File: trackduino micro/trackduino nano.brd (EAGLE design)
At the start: 48.1 x 21.9 mm, 28 parts, among them IC2 74AHC1G125DBV, SW1 SPST_TACT-KMR2, U1 ATMEGA168, Y1 16MHZ

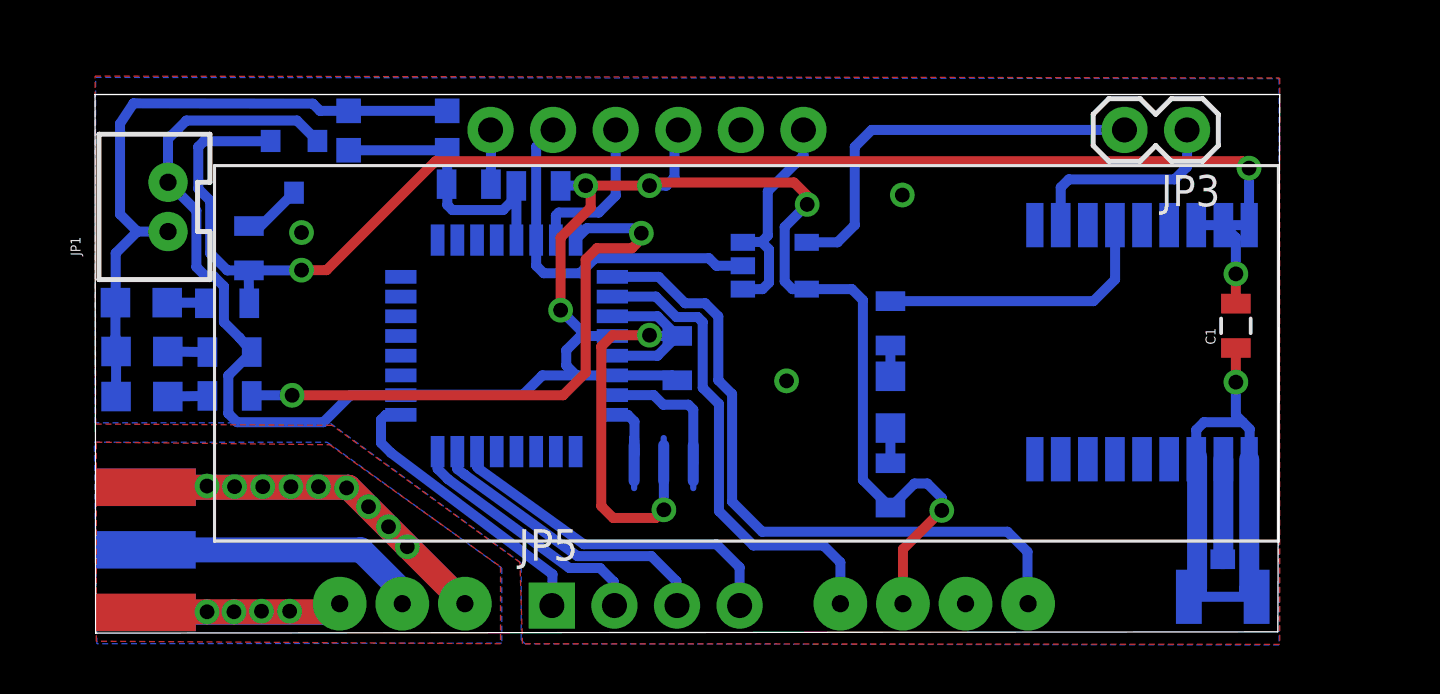
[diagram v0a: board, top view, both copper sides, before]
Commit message: Revert 658c1f1..8864008
This rolls back to commit 658c1f11e5b9c3d0ac6cf8412ef3704af54d539a.
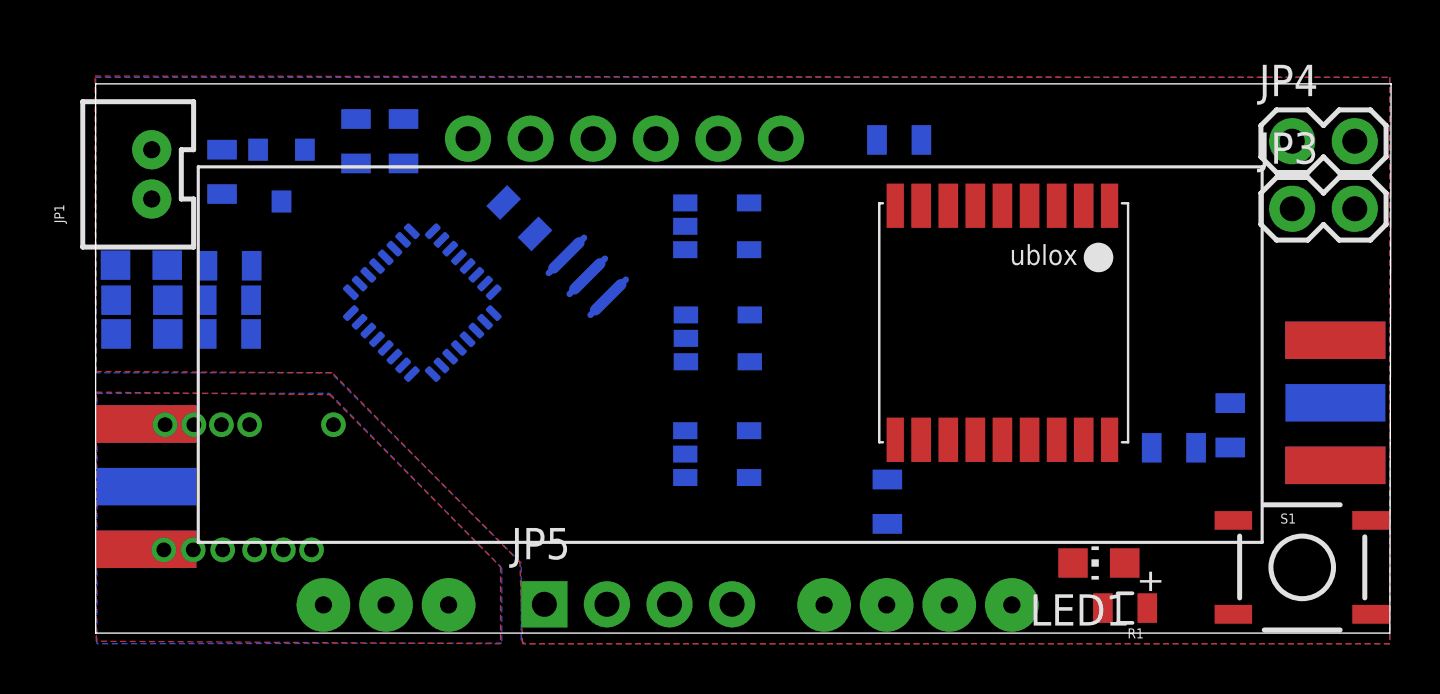
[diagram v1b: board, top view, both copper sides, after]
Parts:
- removed SW1: SPST_TACT-KMR2, adafruit:KMR2
- removed X1: (no value), adafruit:U.FL
- added IC1, IC3: 74AHC1G125DBV, 74xx-little-us:SOT23-5
- added J$2: SMA_EDGE, SparkFun-Connectors:SMA-EDGE
- added JP4: M02PTH, SparkFun-Connectors:1X02
- added L1: (no value), SparkFun-Passives:0805
- added R2: (no value), SparkFun-Resistors:0805
- added S1: TAC_SWITCHSMD, SparkFun-Electromechanical:TACTILE-SWITCH-SMD
- U1: value ATMEGA168 -> ATMEGA168MLF; device SparkFun-DigitalIC:TQFP32-08 -> SparkFun-DigitalIC:MLF32
- moved C1 15.6 mm to (79.3, 77.5), flipped to the bottom, turned to 180 degrees
- moved R1 15.0 mm to (88.4, 58.5), flipped to the top, turned to 180 degrees
- moved LED1 10.7 mm to (87.4, 60.3), flipped to the top, turned to 90 degrees
- moved C3 8.56 mm to (63.9, 74.3), turned to 225 degrees
- moved Y1 8.19 mm to (66.6, 71.9), turned to 225 degrees
- moved R5 7.63 mm to (57.2, 77.4), turned to 90 degrees
- moved U$1 5.82 mm to (83.4, 69.8), flipped to the top
- moved JP3 5.33 mm to (95.2, 74.7), turned to 0 degrees
- moved U1 3.84 mm to (59.9, 70.9), turned to 315 degrees
- moved C2 3.29 mm to (51.8, 76.2), turned to 90 degrees
- moved C5 3.17 mm to (59.2, 77.4), turned to 270 degrees
- moved IC2 2.83 mm to (71.9, 74.0)
- moved J$1 2.57 mm to (48.7, 60.9)
- moved LED4 2.54 mm to (48.5, 69.6)
- moved R6 2.51 mm to (52.1, 69.6)
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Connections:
- new net 7_VCC_IO: U$1.7_VCC_IO
- new net 9_V_RESET: U$1.9_V_RESET
- new net EN-5V: IC3.4, U$2.EN
- new net N$4: R2.1
- new net N$5: L1.1, R2.2
- new net TXD-5V: IC1.4, U$2.TXD
- net 3V: no longer U$1.7_VCC_IO, U$1.9_V_RESET
- net D3: now also IC1.2; no longer U$2.TXD
- net D4: now also IC3.2; no longer U$2.EN
- net GND: now also IC1.1, IC1.3, IC3.1, IC3.3, J$2.GND@0, J$2.GND@1, J$2.GND@2, J$2.GND@3, S1.3, S1.4; no longer SW1.2, SW1.4, X1.1, X1.2
- net N$6: now also J$2.SIG, L1.2; no longer X1.3
- net N$9: now also S1.1, S1.2; no longer SW1.1, SW1.3
- net RX: now also JP4.1
- net RXO: now also JP4.2; no longer IC2.2
- net TX: now also IC2.2
- net TX-3V3: no longer JP3.2
- net TXO: now also JP3.2
- net VCC: now also IC1.5, IC3.5
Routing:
- net GND: track 127.9 -> 0.00 mm, vias 5 -> 0
- net VCC: track 87.9 -> 0.00 mm, vias 5 -> 0
- net 3V: track 61.2 -> 0.00 mm, vias 3 -> 0
- net D3: track 27.7 -> 0.00 mm
- net LED: track 24.3 -> 0.00 mm, vias 2 -> 0
- net D4: track 19.5 -> 0.00 mm
- net TX-3V3: track 16.6 -> 0.00 mm
- net RXO: track 14.7 -> 0.00 mm
- net SS: track 14.2 -> 0.00 mm
- net MOSI: track 12.2 -> 0.00 mm
- net N$9: track 12.0 -> 0.00 mm
- net SCK: track 11.9 -> 0.00 mm
- net N$2: track 11.7 -> 0.00 mm
- net N$1: track 11.6 -> 0.00 mm
- net MISO: track 10.4 -> 0.00 mm
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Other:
- board size 48.1 x 21.9 mm -> 52.6 x 22.3 mm
